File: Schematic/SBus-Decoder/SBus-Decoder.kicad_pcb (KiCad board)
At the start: 2 copper layers, 28.8 x 15.2 mm, 10 parts, among them J1 Conn_01x03_Male, J2 Conn_01x02_Male, J3 TSW-104-08-G-T-RA, U1 PIC18F04Q40-I_ST, U2 MCP1703A-3302_SOT23

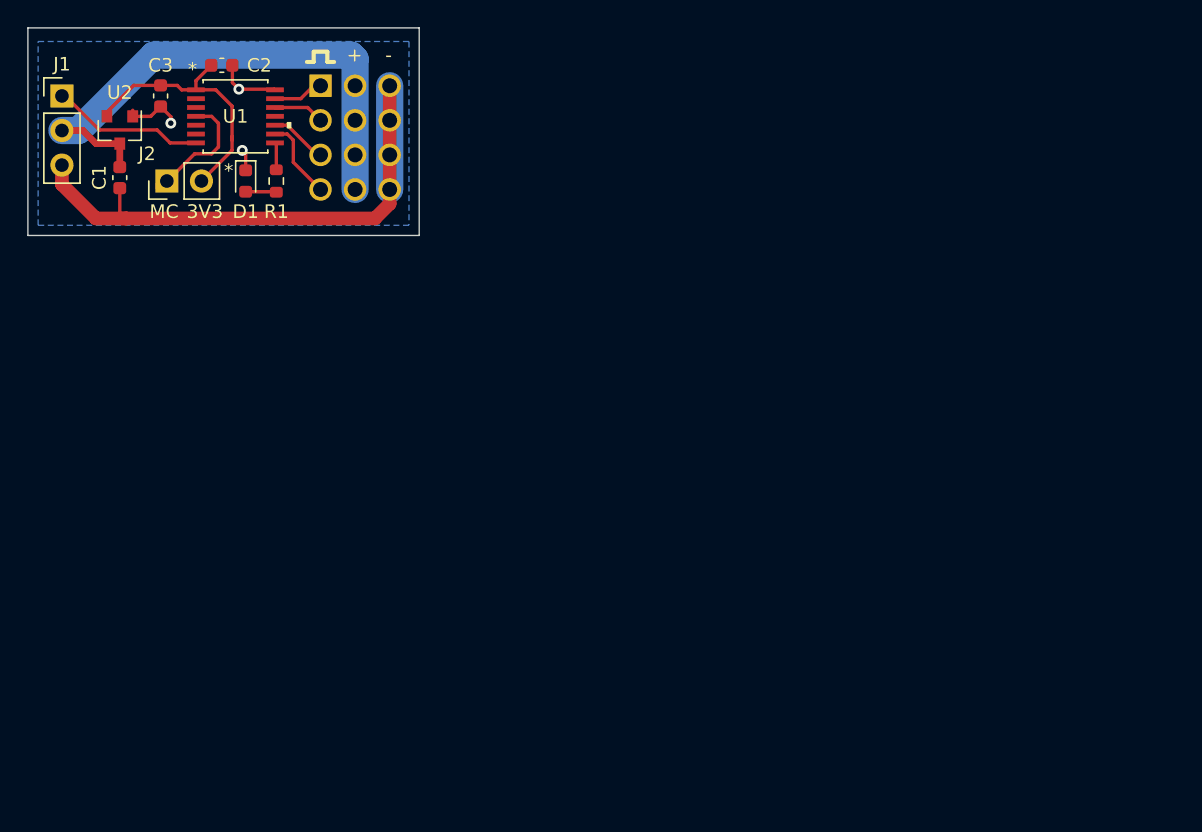
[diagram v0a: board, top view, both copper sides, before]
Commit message: Paneled and generated gerbers
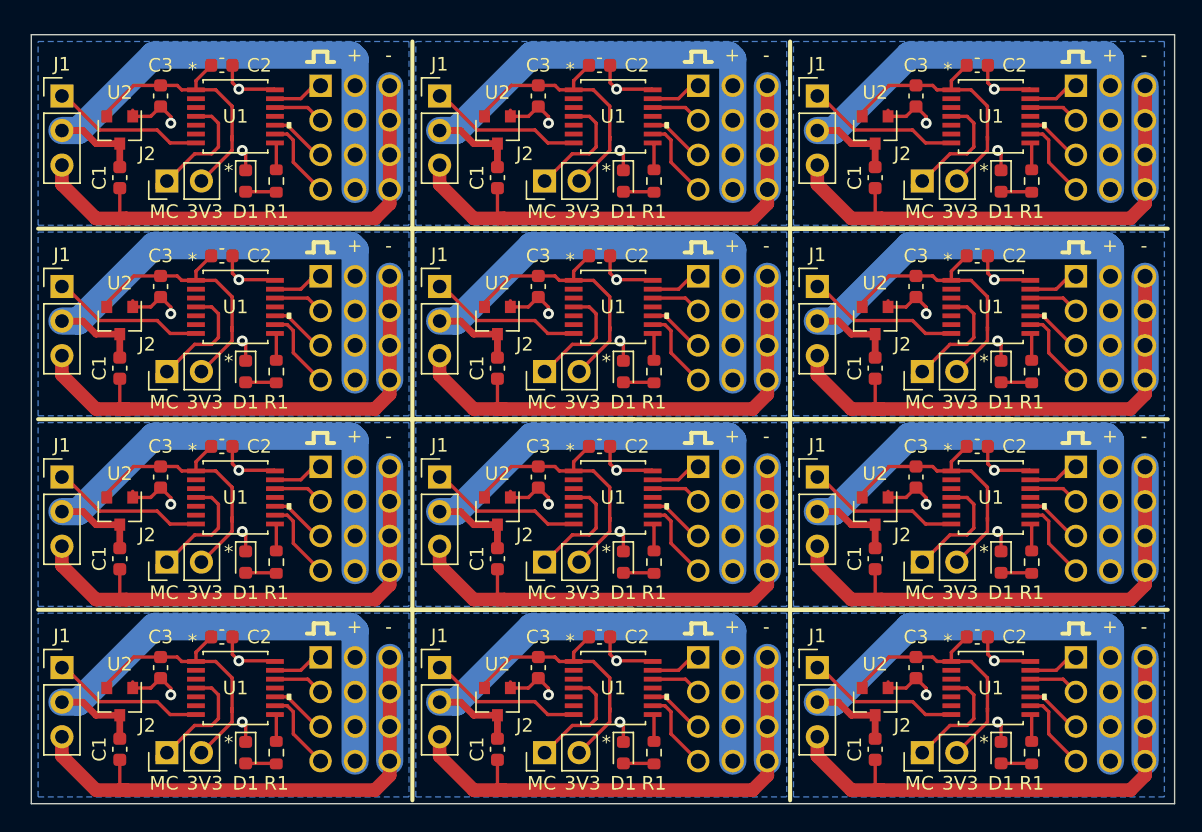
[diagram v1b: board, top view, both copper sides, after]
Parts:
- added C1: 1 uF, Capacitor_SMD:C_0603_1608Metric, F.Cu at (112.2, 88.5)
- added C1: 1 uF, Capacitor_SMD:C_0603_1608Metric, F.Cu at (56.8, 102.5)
- added C1: 1 uF, Capacitor_SMD:C_0603_1608Metric, F.Cu at (56.8, 74.5)
- added C1: 1 uF, Capacitor_SMD:C_0603_1608Metric, F.Cu at (112.2, 102.5)
- added C1: 1 uF, Capacitor_SMD:C_0603_1608Metric, F.Cu at (112.2, 60.5)
- added C1: 1 uF, Capacitor_SMD:C_0603_1608Metric, F.Cu at (112.2, 74.5)
- added C1: 1 uF, Capacitor_SMD:C_0603_1608Metric, F.Cu at (84.5, 88.5)
- added C1: 1 uF, Capacitor_SMD:C_0603_1608Metric, F.Cu at (84.5, 102.5)
- added C1: 1 uF, Capacitor_SMD:C_0603_1608Metric, F.Cu at (84.5, 60.5)
- added C1: 1 uF, Capacitor_SMD:C_0603_1608Metric, F.Cu at (84.5, 74.5)
- added C1: 1 uF, Capacitor_SMD:C_0603_1608Metric, F.Cu at (56.8, 88.5)
- added C2: 0.1 uF, Capacitor_SMD:C_0603_1608Metric, F.Cu at (119.8, 80.2)
- added C2: 0.1 uF, Capacitor_SMD:C_0603_1608Metric, F.Cu at (64.2, 80.2)
- added C2: 0.1 uF, Capacitor_SMD:C_0603_1608Metric, F.Cu at (64.2, 66.2)
- added C2: 0.1 uF, Capacitor_SMD:C_0603_1608Metric, F.Cu at (119.8, 94.2)
- added C2: 0.1 uF, Capacitor_SMD:C_0603_1608Metric, F.Cu at (119.8, 52.2)
- added C2: 0.1 uF, Capacitor_SMD:C_0603_1608Metric, F.Cu at (119.8, 66.2)
- added C2: 0.1 uF, Capacitor_SMD:C_0603_1608Metric, F.Cu at (92.0, 94.2)
- added C2: 0.1 uF, Capacitor_SMD:C_0603_1608Metric, F.Cu at (92.0, 80.2)
- added C2: 0.1 uF, Capacitor_SMD:C_0603_1608Metric, F.Cu at (92.0, 66.2)
- added C2: 0.1 uF, Capacitor_SMD:C_0603_1608Metric, F.Cu at (92.0, 52.2)
- added C2: 0.1 uF, Capacitor_SMD:C_0603_1608Metric, F.Cu at (64.2, 94.2)
- added C3: 2.2 uF, Capacitor_SMD:C_0603_1608Metric, F.Cu at (115.2, 96.5)
- added C3: 2.2 uF, Capacitor_SMD:C_0603_1608Metric, F.Cu at (59.8, 96.5)
- added C3: 2.2 uF, Capacitor_SMD:C_0603_1608Metric, F.Cu at (59.8, 68.5)
- added C3: 2.2 uF, Capacitor_SMD:C_0603_1608Metric, F.Cu at (115.2, 82.5)
- added C3: 2.2 uF, Capacitor_SMD:C_0603_1608Metric, F.Cu at (115.2, 54.5)
- added C3: 2.2 uF, Capacitor_SMD:C_0603_1608Metric, F.Cu at (115.2, 68.5)
- added C3: 2.2 uF, Capacitor_SMD:C_0603_1608Metric, F.Cu at (87.5, 96.5)
- added C3: 2.2 uF, Capacitor_SMD:C_0603_1608Metric, F.Cu at (87.5, 82.5)
- added C3: 2.2 uF, Capacitor_SMD:C_0603_1608Metric, F.Cu at (87.5, 54.5)
- added C3: 2.2 uF, Capacitor_SMD:C_0603_1608Metric, F.Cu at (87.5, 68.5)
- added C3: 2.2 uF, Capacitor_SMD:C_0603_1608Metric, F.Cu at (59.8, 82.5)
- added D1: LED-Red, LED_SMD:LED_0603_1608Metric, F.Cu at (121.5, 102.8)
- added D1: LED-Red, LED_SMD:LED_0603_1608Metric, F.Cu at (66.0, 102.8)
- added D1: LED-Red, LED_SMD:LED_0603_1608Metric, F.Cu at (66.0, 74.8)
- added D1: LED-Red, LED_SMD:LED_0603_1608Metric, F.Cu at (121.5, 74.8)
- added D1: LED-Red, LED_SMD:LED_0603_1608Metric, F.Cu at (121.5, 60.8)
- added D1: LED-Red, LED_SMD:LED_0603_1608Metric, F.Cu at (121.5, 88.8)
- added D1: LED-Red, LED_SMD:LED_0603_1608Metric, F.Cu at (93.8, 60.8)
- added D1: LED-Red, LED_SMD:LED_0603_1608Metric, F.Cu at (93.8, 102.8)
- added D1: LED-Red, LED_SMD:LED_0603_1608Metric, F.Cu at (93.8, 74.8)
- added D1: LED-Red, LED_SMD:LED_0603_1608Metric, F.Cu at (93.8, 88.8)
- added D1: LED-Red, LED_SMD:LED_0603_1608Metric, F.Cu at (66.0, 88.8)
- added J1: Conn_01x03_Male, Connector_PinHeader_2.54mm:PinHeader_1x03_P2.54mm_Vertical, F.Cu at (108.0, 68.5)
- added J1: Conn_01x03_Male, Connector_PinHeader_2.54mm:PinHeader_1x03_P2.54mm_Vertical, F.Cu at (52.5, 96.5)
- added J1: Conn_01x03_Male, Connector_PinHeader_2.54mm:PinHeader_1x03_P2.54mm_Vertical, F.Cu at (52.5, 68.5)
- added J1: Conn_01x03_Male, Connector_PinHeader_2.54mm:PinHeader_1x03_P2.54mm_Vertical, F.Cu at (108.0, 54.5)
- added J1: Conn_01x03_Male, Connector_PinHeader_2.54mm:PinHeader_1x03_P2.54mm_Vertical, F.Cu at (108.0, 82.5)
- added J1: Conn_01x03_Male, Connector_PinHeader_2.54mm:PinHeader_1x03_P2.54mm_Vertical, F.Cu at (108.0, 96.5)
- added J1: Conn_01x03_Male, Connector_PinHeader_2.54mm:PinHeader_1x03_P2.54mm_Vertical, F.Cu at (80.2, 54.5)
- added J1: Conn_01x03_Male, Connector_PinHeader_2.54mm:PinHeader_1x03_P2.54mm_Vertical, F.Cu at (80.2, 68.5)
- added J1: Conn_01x03_Male, Connector_PinHeader_2.54mm:PinHeader_1x03_P2.54mm_Vertical, F.Cu at (80.2, 82.5)
- added J1: Conn_01x03_Male, Connector_PinHeader_2.54mm:PinHeader_1x03_P2.54mm_Vertical, F.Cu at (80.2, 96.5)
- added J1: Conn_01x03_Male, Connector_PinHeader_2.54mm:PinHeader_1x03_P2.54mm_Vertical, F.Cu at (52.5, 82.5)
- added J2: Conn_01x02_Male, Connector_PinHeader_2.54mm:PinHeader_1x02_P2.54mm_Vertical, F.Cu at (115.7, 102.8)
- added J2: Conn_01x02_Male, Connector_PinHeader_2.54mm:PinHeader_1x02_P2.54mm_Vertical, F.Cu at (60.2, 88.8)
- added J2: Conn_01x02_Male, Connector_PinHeader_2.54mm:PinHeader_1x02_P2.54mm_Vertical, F.Cu at (60.2, 74.8)
- added J2: Conn_01x02_Male, Connector_PinHeader_2.54mm:PinHeader_1x02_P2.54mm_Vertical, F.Cu at (115.7, 88.8)
- added J2: Conn_01x02_Male, Connector_PinHeader_2.54mm:PinHeader_1x02_P2.54mm_Vertical, F.Cu at (115.7, 60.8)
- added J2: Conn_01x02_Male, Connector_PinHeader_2.54mm:PinHeader_1x02_P2.54mm_Vertical, F.Cu at (115.7, 74.8)
- added J2: Conn_01x02_Male, Connector_PinHeader_2.54mm:PinHeader_1x02_P2.54mm_Vertical, F.Cu at (88.0, 88.8)
- added J2: Conn_01x02_Male, Connector_PinHeader_2.54mm:PinHeader_1x02_P2.54mm_Vertical, F.Cu at (88.0, 102.8)
- added J2: Conn_01x02_Male, Connector_PinHeader_2.54mm:PinHeader_1x02_P2.54mm_Vertical, F.Cu at (88.0, 74.8)
- added J2: Conn_01x02_Male, Connector_PinHeader_2.54mm:PinHeader_1x02_P2.54mm_Vertical, F.Cu at (88.0, 60.8)
- added J2: Conn_01x02_Male, Connector_PinHeader_2.54mm:PinHeader_1x02_P2.54mm_Vertical, F.Cu at (60.2, 102.8)
- added J3: TSW-104-08-G-T-RA, SamacSys_Parts:HDRRA12W64P254_3X4_1016X254X810P, F.Cu at (127.0, 67.8)
- added J3: TSW-104-08-G-T-RA, SamacSys_Parts:HDRRA12W64P254_3X4_1016X254X810P, F.Cu at (71.5, 95.8)
- added J3: TSW-104-08-G-T-RA, SamacSys_Parts:HDRRA12W64P254_3X4_1016X254X810P, F.Cu at (71.5, 67.8)
- added J3: TSW-104-08-G-T-RA, SamacSys_Parts:HDRRA12W64P254_3X4_1016X254X810P, F.Cu at (127.0, 95.8)
- added J3: TSW-104-08-G-T-RA, SamacSys_Parts:HDRRA12W64P254_3X4_1016X254X810P, F.Cu at (127.0, 53.8)
- added J3: TSW-104-08-G-T-RA, SamacSys_Parts:HDRRA12W64P254_3X4_1016X254X810P, F.Cu at (127.0, 81.8)
- added J3: TSW-104-08-G-T-RA, SamacSys_Parts:HDRRA12W64P254_3X4_1016X254X810P, F.Cu at (99.2, 53.8)
- added J3: TSW-104-08-G-T-RA, SamacSys_Parts:HDRRA12W64P254_3X4_1016X254X810P, F.Cu at (99.2, 95.8)
- added J3: TSW-104-08-G-T-RA, SamacSys_Parts:HDRRA12W64P254_3X4_1016X254X810P, F.Cu at (99.2, 67.8)
- added J3: TSW-104-08-G-T-RA, SamacSys_Parts:HDRRA12W64P254_3X4_1016X254X810P, F.Cu at (99.2, 81.8)
- added J3: TSW-104-08-G-T-RA, SamacSys_Parts:HDRRA12W64P254_3X4_1016X254X810P, F.Cu at (71.5, 81.8)
- added R1: 220, Resistor_SMD:R_0603_1608Metric, F.Cu at (123.8, 74.8)
- added R1: 220, Resistor_SMD:R_0603_1608Metric, F.Cu at (68.2, 102.8)
- added R1: 220, Resistor_SMD:R_0603_1608Metric, F.Cu at (68.2, 74.8)
- added R1: 220, Resistor_SMD:R_0603_1608Metric, F.Cu at (123.8, 60.8)
- added R1: 220, Resistor_SMD:R_0603_1608Metric, F.Cu at (123.8, 102.8)
- added R1: 220, Resistor_SMD:R_0603_1608Metric, F.Cu at (123.8, 88.8)
- added R1: 220, Resistor_SMD:R_0603_1608Metric, F.Cu at (96.0, 60.8)
- added R1: 220, Resistor_SMD:R_0603_1608Metric, F.Cu at (96.0, 74.8)
- added R1: 220, Resistor_SMD:R_0603_1608Metric, F.Cu at (96.0, 88.8)
- added R1: 220, Resistor_SMD:R_0603_1608Metric, F.Cu at (96.0, 102.8)
- added R1: 220, Resistor_SMD:R_0603_1608Metric, F.Cu at (68.2, 88.8)
- added U1: PIC18F04Q40-I_ST, PIC18F0xQ40:PIC18F04Q40-I&slash_ST, F.Cu at (120.8, 98.0)
- added U1: PIC18F04Q40-I_ST, PIC18F0xQ40:PIC18F04Q40-I&slash_ST, F.Cu at (65.2, 84.0)
- added U1: PIC18F04Q40-I_ST, PIC18F0xQ40:PIC18F04Q40-I&slash_ST, F.Cu at (65.2, 70.0)
- added U1: PIC18F04Q40-I_ST, PIC18F0xQ40:PIC18F04Q40-I&slash_ST, F.Cu at (120.8, 84.0)
- added U1: PIC18F04Q40-I_ST, PIC18F0xQ40:PIC18F04Q40-I&slash_ST, F.Cu at (120.8, 56.0)
- added U1: PIC18F04Q40-I_ST, PIC18F0xQ40:PIC18F04Q40-I&slash_ST, F.Cu at (120.8, 70.0)
- added U1: PIC18F04Q40-I_ST, PIC18F0xQ40:PIC18F04Q40-I&slash_ST, F.Cu at (93.0, 98.0)
- added U1: PIC18F04Q40-I_ST, PIC18F0xQ40:PIC18F04Q40-I&slash_ST, F.Cu at (93.0, 84.0)
- added U1: PIC18F04Q40-I_ST, PIC18F0xQ40:PIC18F04Q40-I&slash_ST, F.Cu at (93.0, 70.0)
- added U1: PIC18F04Q40-I_ST, PIC18F0xQ40:PIC18F04Q40-I&slash_ST, F.Cu at (93.0, 56.0)
- added U1: PIC18F04Q40-I_ST, PIC18F0xQ40:PIC18F04Q40-I&slash_ST, F.Cu at (65.2, 98.0)
- added U2: MCP1703A-3302_SOT23, Package_TO_SOT_SMD:SOT-23, F.Cu at (112.2, 85.0)
- added U2: MCP1703A-3302_SOT23, Package_TO_SOT_SMD:SOT-23, F.Cu at (56.8, 85.0)
- added U2: MCP1703A-3302_SOT23, Package_TO_SOT_SMD:SOT-23, F.Cu at (56.8, 71.0)
- added U2: MCP1703A-3302_SOT23, Package_TO_SOT_SMD:SOT-23, F.Cu at (112.2, 99.0)
- added U2: MCP1703A-3302_SOT23, Package_TO_SOT_SMD:SOT-23, F.Cu at (112.2, 57.0)
- added U2: MCP1703A-3302_SOT23, Package_TO_SOT_SMD:SOT-23, F.Cu at (112.2, 71.0)
- added U2: MCP1703A-3302_SOT23, Package_TO_SOT_SMD:SOT-23, F.Cu at (84.5, 85.0)
- added U2: MCP1703A-3302_SOT23, Package_TO_SOT_SMD:SOT-23, F.Cu at (84.5, 99.0)
- added U2: MCP1703A-3302_SOT23, Package_TO_SOT_SMD:SOT-23, F.Cu at (84.5, 71.0)
- added U2: MCP1703A-3302_SOT23, Package_TO_SOT_SMD:SOT-23, F.Cu at (84.5, 57.0)
- added U2: MCP1703A-3302_SOT23, Package_TO_SOT_SMD:SOT-23, F.Cu at (56.8, 99.0)
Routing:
- net GND: track 56.6 -> 679.5 mm, vias 3 -> 36
- net VBUS: track 40.6 -> 487.4 mm
- net +3V3: track 19.9 -> 238.8 mm
- net Net-(J1-Pad1): track 11.3 -> 135.3 mm
- net Net-(J2-Pad1): track 8.93 -> 107.2 mm
- net Net-(J3-Pad10): track 5.99 -> 71.8 mm
- net Net-(J3-Pad7): track 4.25 -> 51.0 mm
- net Net-(J3-Pad1): track 3.74 -> 44.9 mm
- net Net-(J3-Pad4): track 3.74 -> 44.8 mm
- net Net-(D1-Pad2): track 2.27 -> 27.2 mm
- net Net-(R1-Pad2): track 2.02 -> 24.2 mm
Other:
- board size 28.8 x 15.2 mm -> 84 x 56.5 mm
- board text added: "JLCJLCJLCJLC"
